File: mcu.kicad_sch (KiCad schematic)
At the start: 4 parts, among them U7 ADA3708

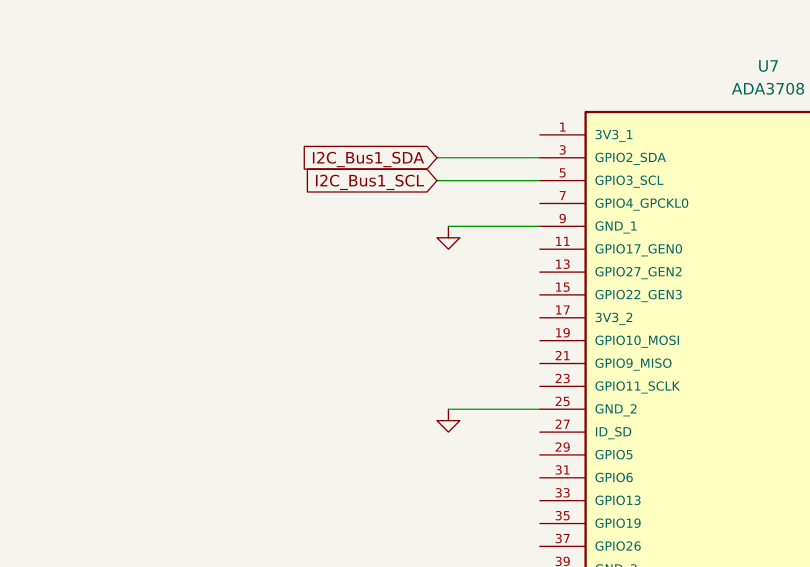
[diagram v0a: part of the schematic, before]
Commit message: routing
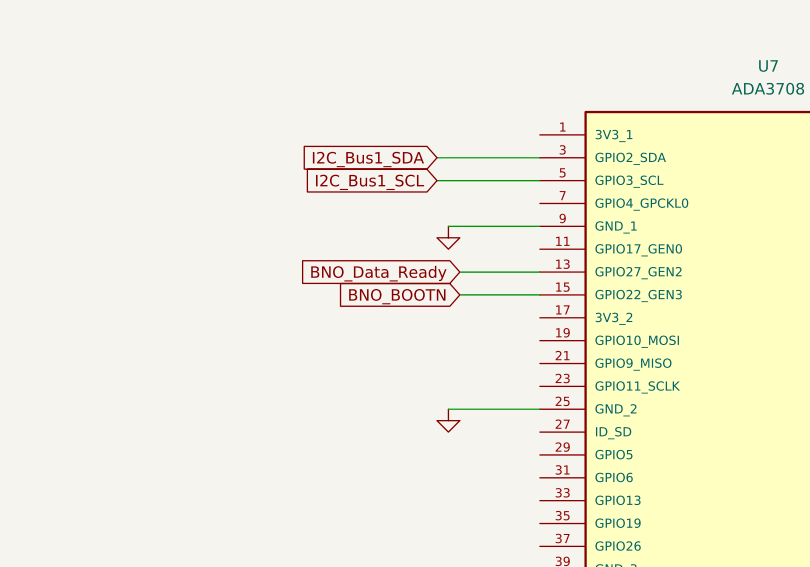
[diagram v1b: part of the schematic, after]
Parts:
- C16, C17, C18: footprint (none) -> Capacitor_SMD:C_0603_1608Metric_Pad1.08x0.95mm_HandSolder
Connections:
- net BNO_Data_Ready: now reaches U7.13 (GPIO27_GEN2)
- net BNO_BOOTN: now reaches U7.15 (GPIO22_GEN3)
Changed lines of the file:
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@@
+    (stroke (width 0) (type default))
+  )
+  (wire (pts (xy 118.11 83.82) (xy 127 83.82))
     (stroke (width 0) (type default))
   )
@@
   )
   (wire (pts (xy 115.57 73.66) (xy 127 73.66))
+    (stroke (width 0) (type default))
+  )
+  (wire (pts (xy 118.11 86.36) (xy 127 86.36))
     (stroke (width 0) (type default))
   )
@@
     )
   )
+  (global_label "BNO_Data_Ready" (shape input) (at 118.11 83.82 180) (fields_autoplaced)
+    (effects (font (size 1.27 1.27)) (justify right))
+    (property "Intersheetrefs" "${INTERSHEET_REFS}" (at 99.4201 83.82 0)
+      (effects (font (size 1.27 1.27)) (justify right) hide)
+    )
+  )
   (global_label "+5v" (shape input) (at 69.85 25.4 0) (fields_autoplaced)
     (effects (font (size 1.27 1.27)) (justify left))
@@
     (effects (font (size 1.27 1.27)) (justify right))
     (property "Intersheetrefs" "${INTERSHEET_REFS}" (at 99.4805 73.66 0)
+      (effects (font (size 1.27 1.27)) (justify right) hide)
+    )
+  )
+  (global_label "BNO_BOOTN" (shape input) (at 118.11 86.36 180) (fields_autoplaced)
+    (effects (font (size 1.27 1.27)) (justify right))
+    (property "Intersheetrefs" "${INTERSHEET_REFS}" (at 104.0765 86.36 0)
       (effects (font (size 1.27 1.27)) (justify right) hide)
     )
@@
       (effects (font (size 1.27 1.27)) (justify left))
     )
-    (property "Footprint" "" (at 36.5252 33.02 0)
+    (property "Footprint" "Capacitor_SMD:C_0603_1608Metric_Pad1.08x0.95mm_HandSolder" (at 36.5252 33.02 0)
       (effects (font (size 1.27 1.27)) hide)
     )
@@
       (effects (font (size 1.27 1.27)) (justify left))
     )
-    (property "Footprint" "" (at 49.2252 33.02 0)
+    (property "Footprint" "Capacitor_SMD:C_0603_1608Metric_Pad1.08x0.95mm_HandSolder" (at 49.2252 33.02 0)
       (effects (font (size 1.27 1.27)) hide)
     )
@@
       (effects (font (size 1.27 1.27)) (justify left))
     )
-    (property "Footprint" "" (at 60.6552 33.02 0)
-      (effects (font (size 1.27 1.27)) hide)
-    )
+    (property "Footprint" "Capacitor_SMD:C_0603_1608Metric_Pad1.08x0.95mm_HandSolder" (at 60.6552 33.02 0)
+      (effects (font (size 1.27 1.27)) hide)
+    )
